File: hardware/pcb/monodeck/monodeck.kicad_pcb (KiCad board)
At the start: 2 copper layers, 71 x 53.8 mm, 14 parts, among them J1 Conn_01x20_Socket, J2 Conn_01x20_Socket, U1 TP4056

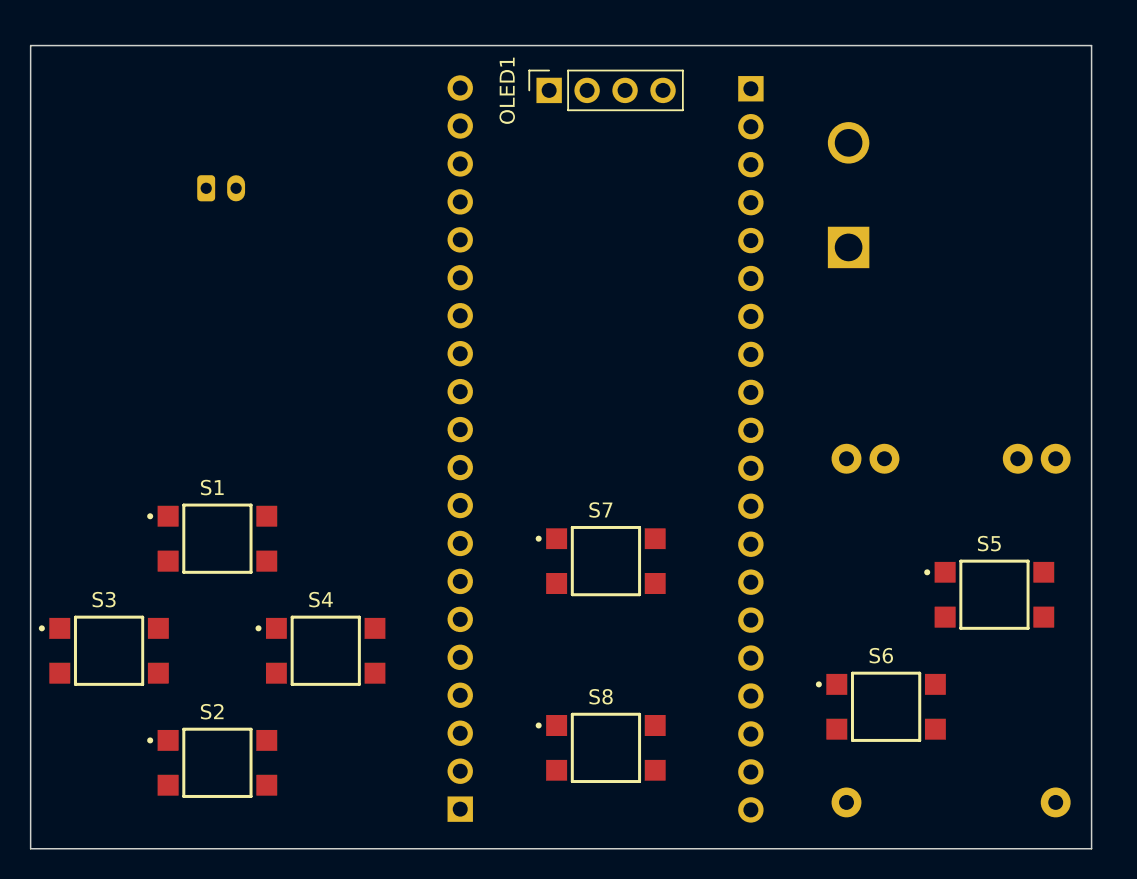
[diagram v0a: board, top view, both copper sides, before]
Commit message: finished first iteration of pcb
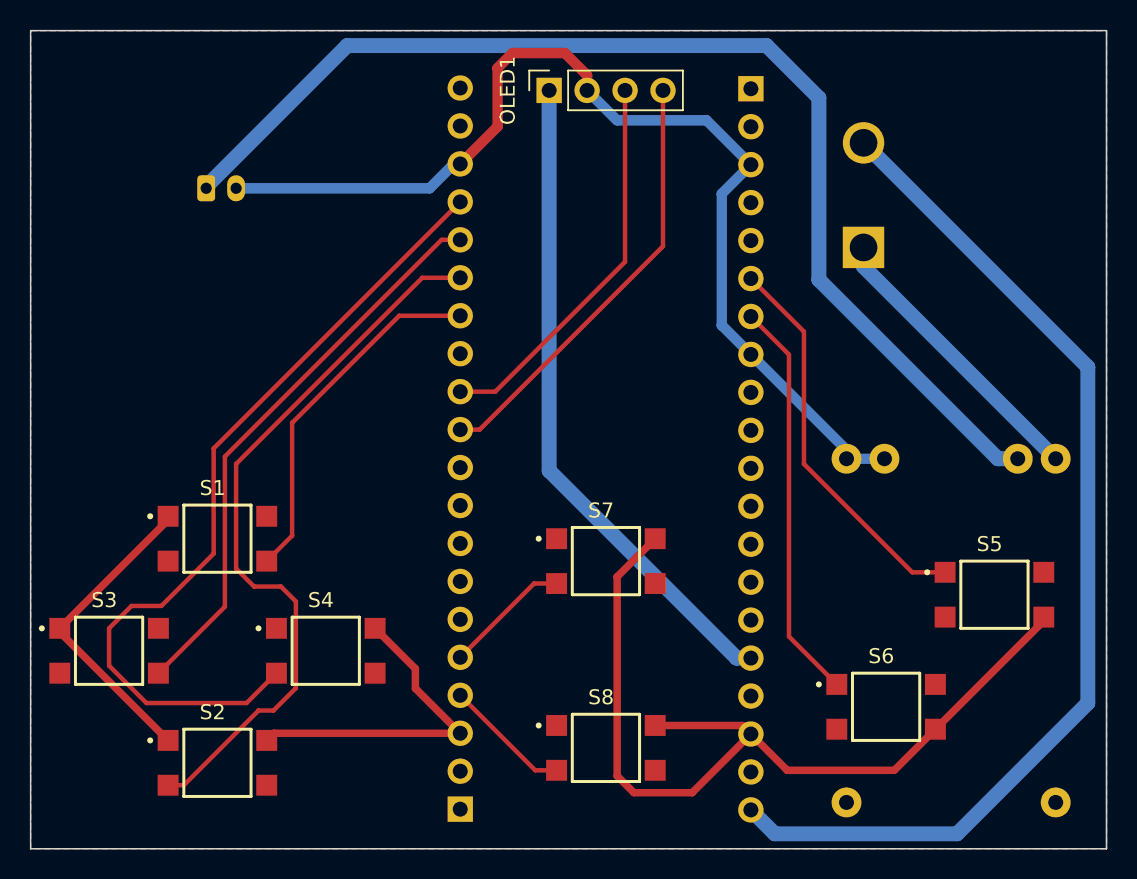
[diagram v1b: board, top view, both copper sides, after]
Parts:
- moved PWR1 1.00 mm to (184.5, 65.5)
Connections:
- J1 pad 13: GND -> unconnected-(J1-GND-Pad13)
- J1 pad 3: GND -> GND1
- J1 pad 4: unconnected-(J1-GP2-Pad4) -> /GPIO2
- J1 pad 5: unconnected-(J1-GP3-Pad5) -> /GPIO3
- J1 pad 8: GND -> unconnected-(J1-GND-Pad8)
- J2 pad 13: GND -> unconnected-(J2-GND-Pad13)
- J2 pad 18: GND -> GND2
- S1 pad 1: unconnected-(S1-Pad1) -> GND1
- S1 pad 2: GND -> unconnected-(S1-Pad2)
- S2 pad 1: unconnected-(S2-Pad1) -> GND1
- S2 pad 2: GND -> GND1
- S2 pad 3: unconnected-(S2-Pad3) -> /GPIO11
- S2 pad 4: /GPIO11 -> unconnected-(S2-Pad4)
- S3 pad 1: unconnected-(S3-Pad1) -> GND1
- S3 pad 2: GND -> unconnected-(S3-Pad2)
- S4 pad 2: GND -> GND1
- S4 pad 3: unconnected-(S4-Pad3) -> /GPIO13
- S4 pad 4: /GPIO13 -> unconnected-(S4-Pad4)
- S5 pad 1: unconnected-(S5-Pad1) -> /GPIO20
- S5 pad 2: /GPIO14 -> unconnected-(S5-Pad2)
- S5 pad 4: GND -> GND2
- S6 pad 1: unconnected-(S6-Pad1) -> /GPIO21
- S6 pad 2: /GPIO15 -> unconnected-(S6-Pad2)
- S6 pad 4: GND -> GND2
- S7 pad 2: GND -> GND2
- S7 pad 3: unconnected-(S7-Pad3) -> /GPIO3
- S7 pad 4: /GPIO20 -> unconnected-(S7-Pad4)
- S8 pad 2: GND -> GND2
- S8 pad 3: unconnected-(S8-Pad3) -> /GPIO2
- S8 pad 4: /GPIO21 -> unconnected-(S8-Pad4)
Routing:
- net Net-(BAT1-Pin_1): track 0.00 -> 76.9 mm
- net GND: track 0.00 -> 70.7 mm
- net /V+: track 0.00 -> 70.5 mm
- net GND2: track 0.00 -> 59.6 mm
- net /GPIO13: track 0.00 -> 55.0 mm
- net /GPIO11: track 0.00 -> 49.1 mm
- net /VCC: track 0.00 -> 44.1 mm
- net GND1: track 0.00 -> 43.8 mm
- net /GPIO12: track 0.00 -> 38.1 mm
- net /GPIO8: track 0.00 -> 29.1 mm
- net /GPIO21: track 0.00 -> 27.0 mm
- net /GPIO20: track 0.00 -> 26.3 mm
- net /GPIO9: track 0.00 -> 26.1 mm
- net /GPIO10: track 0.00 -> 24.2 mm
- net Net-(U1-Vout+): track 0.00 -> 19.5 mm
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- added copper zone on B.Cu, net GND
- added copper zone on F.Cu, net GND
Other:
- board size 71 x 53.8 mm -> 72 x 54.8 mm
